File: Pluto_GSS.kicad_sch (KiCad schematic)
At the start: 7 parts

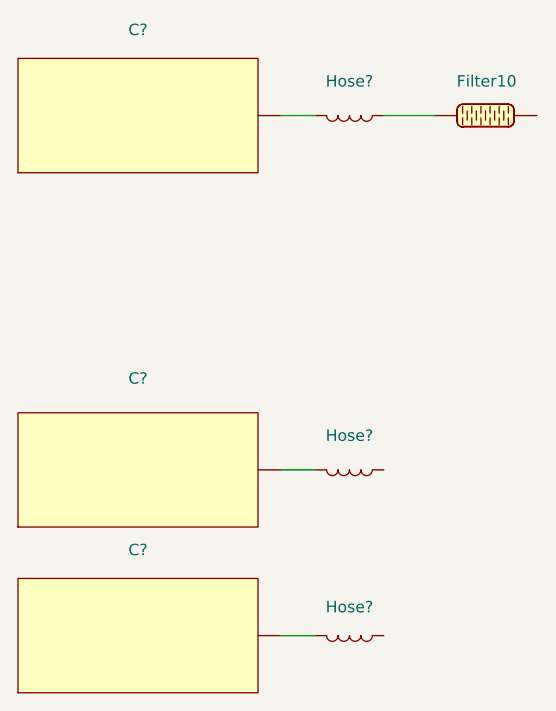
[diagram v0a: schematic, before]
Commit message: Formatiing
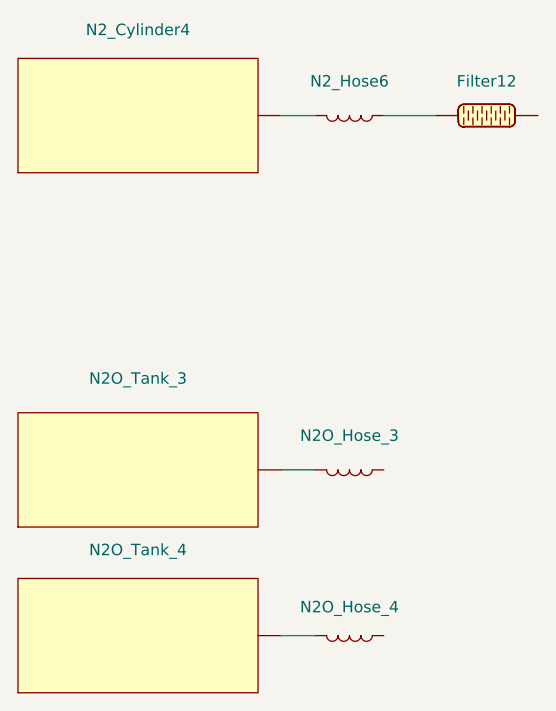
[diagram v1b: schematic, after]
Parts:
- gave numbers to parts that had none: 6
- renumbered Filter10 to Filter12
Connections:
- net at N2O_Hose_4.: now also N2O_Tank_4.
- net at Filter12.: now also N2_Hose6.
- net at N2_Hose6.: now also N2_Cylinder4.
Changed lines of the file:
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@@
 		(dnp no)
 		(fields_autoplaced yes)
-		(property "Reference" "C?"
+		(property "Reference" "N2O_Tank_3"
 			(at 77.47 93.98 90)
 			(effects
@@
 					(size 1.27 1.27)
 				)
-				(hide yes)
 			)
 		)
@@
 					(size 1.27 1.27)
 				)
-			)
-		)
-		(pin ""
-		)
-		(instances
-			(project "P_IDs"
-				(path "/045f1f05-3134-4b6d-91b6-463031104f1e/d4c68d07-3148-4b28-9ebc-772298248340/d1c23521-1854-4751-80d3-fa4616e29f0e"
-					(reference "C?")
-					(unit 1)
-				)
-			)
-		)
-	)
-	(symbol
+				(hide yes)
+			)
+		)
+		(pin ""
+		)
+		(instances
+			(project "P_IDs"
+				(path "/045f1f05-3134-4b6d-91b6-463031104f1e/d4c68d07-3148-4b28-9ebc-772298248340/d1c23521-1854-4751-80d3-fa4616e29f0e"
+					(reference "N2O_Tank_3")
+					(unit 1)
+				)
+			)
+		)
+	)
+	(symbol
+		(lib_name "Hose_1")
 		(lib_id "PID_symbols:Hose")
 		(at 97.155 122.555 270)
@@
 		(dnp no)
 		(fields_autoplaced yes)
-		(property "Reference" "Hose?"
+		(property "Reference" "N2O_Hose_4"
 			(at 100.965 119.38 90)
 			(effects
@@
 					(size 1.27 1.27)
 				)
-				(hide yes)
 			)
 		)
@@
 					(size 1.27 1.27)
 				)
-			)
-		)
-		(pin ""
-		)
-		(pin ""
-		)
-		(instances
-			(project "P_IDs"
-				(path "/045f1f05-3134-4b6d-91b6-463031104f1e/d4c68d07-3148-4b28-9ebc-772298248340/d1c23521-1854-4751-80d3-fa4616e29f0e"
-					(reference "Hose?")
+				(hide yes)
+			)
+		)
+		(pin ""
+		)
+		(pin ""
+		)
+		(instances
+			(project "P_IDs"
+				(path "/045f1f05-3134-4b6d-91b6-463031104f1e/d4c68d07-3148-4b28-9ebc-772298248340/d1c23521-1854-4751-80d3-fa4616e29f0e"
+					(reference "N2O_Hose_4")
 					(unit 1)
 				)
@@
 		(on_board yes)
 		(dnp no)
-		(property "Reference" "Filter10"
+		(property "Reference" "Filter12"
 			(at 116.205 60.96 0)
 			(effects
@@
 					(size 1.27 1.27)
 				)
-				(hide yes)
 			)
 		)
@@
 					(size 1.27 1.27)
 				)
-			)
-		)
-		(pin ""
-		)
-		(pin ""
-		)
-		(instances
-			(project "P_IDs"
-				(path "/045f1f05-3134-4b6d-91b6-463031104f1e/d4c68d07-3148-4b28-9ebc-772298248340/d1c23521-1854-4751-80d3-fa4616e29f0e"
-					(reference "Filter10")
+				(hide yes)
+			)
+		)
+		(pin ""
+		)
+		(pin ""
+		)
+		(instances
+			(project "P_IDs"
+				(path "/045f1f05-3134-4b6d-91b6-463031104f1e/d4c68d07-3148-4b28-9ebc-772298248340/d1c23521-1854-4751-80d3-fa4616e29f0e"
+					(reference "Filter12")
 					(unit 1)
 				)
@@
 		(dnp no)
 		(fields_autoplaced yes)
-		(property "Reference" "C?"
+		(property "Reference" "N2O_Tank_4"
 			(at 77.47 113.03 90)
 			(effects
@@
 					(size 1.27 1.27)
 				)
-				(hide yes)
 			)
 		)
@@
 					(size 1.27 1.27)
 				)
-			)
-		)
-		(pin ""
-		)
-		(instances
-			(project "P_IDs"
-				(path "/045f1f05-3134-4b6d-91b6-463031104f1e/d4c68d07-3148-4b28-9ebc-772298248340/d1c23521-1854-4751-80d3-fa4616e29f0e"
-					(reference "C?")
-					(unit 1)
-				)
-			)
-		)
-	)
-	(symbol
-		(lib_name "Hose_1")
+				(hide yes)
+			)
+		)
+		(pin ""
+		)
+		(instances
+			(project "P_IDs"
+				(path "/045f1f05-3134-4b6d-91b6-463031104f1e/d4c68d07-3148-4b28-9ebc-772298248340/d1c23521-1854-4751-80d3-fa4616e29f0e"
+					(reference "N2O_Tank_4")
+					(unit 1)
+				)
+			)
+		)
+	)
+	(symbol
 		(lib_id "PID_symbols:Hose")
 		(at 97.155 104.14 270)
@@
 		(dnp no)
 		(fields_autoplaced yes)
-		(property "Reference" "Hose?"
+		(property "Reference" "N2O_Hose_3"
 			(at 100.965 100.33 90)
 			(effects
@@
 					(size 1.27 1.27)
 				)
-				(hide yes)
 			)
 		)
@@
 					(size 1.27 1.27)
 				)
-			)
-		)
-		(pin ""
-		)
-		(pin ""
-		)
-		(instances
-			(project "P_IDs"
-				(path "/045f1f05-3134-4b6d-91b6-463031104f1e/d4c68d07-3148-4b28-9ebc-772298248340/d1c23521-1854-4751-80d3-fa4616e29f0e"
-					(reference "Hose?")
+				(hide yes)
+			)
+		)
+		(pin ""
+		)
+		(pin ""
+		)
+		(instances
+			(project "P_IDs"
+				(path "/045f1f05-3134-4b6d-91b6-463031104f1e/d4c68d07-3148-4b28-9ebc-772298248340/d1c23521-1854-4751-80d3-fa4616e29f0e"
+					(reference "N2O_Hose_3")
 					(unit 1)
 				)
@@
 		(dnp no)
 		(fields_autoplaced yes)
-		(property "Reference" "Hose?"
+		(property "Reference" "N2_Hose6"
 			(at 100.965 60.96 90)
 			(effects
@@
 					(size 1.27 1.27)
 				)
-				(hide yes)
 			)
 		)
@@
 					(size 1.27 1.27)
 				)
-			)
-		)
-		(pin ""
-		)
-		(pin ""
-		)
-		(instances
-			(project "P_IDs"
-				(path "/045f1f05-3134-4b6d-91b6-463031104f1e/d4c68d07-3148-4b28-9ebc-772298248340/d1c23521-1854-4751-80d3-fa4616e29f0e"
-					(reference "Hose?")
+				(hide yes)
+			)
+		)
+		(pin ""
+		)
+		(pin ""
+		)
+		(instances
+			(project "P_IDs"
+				(path "/045f1f05-3134-4b6d-91b6-463031104f1e/d4c68d07-3148-4b28-9ebc-772298248340/d1c23521-1854-4751-80d3-fa4616e29f0e"
+					(reference "N2_Hose6")
 					(unit 1)
 				)
@@
 		(dnp no)
 		(fields_autoplaced yes)
-		(property "Reference" "C?"
+		(property "Reference" "N2_Cylinder4"
 			(at 77.47 55.245 90)
 			(effects
@@
 					(size 1.27 1.27)
 				)
-				(hide yes)
 			)
 		)
@@
 					(size 1.27 1.27)
 				)
-			)
-		)
-		(pin ""
-		)
-		(instances
-			(project "P_IDs"
-				(path "/045f1f05-3134-4b6d-91b6-463031104f1e/d4c68d07-3148-4b28-9ebc-772298248340/d1c23521-1854-4751-80d3-fa4616e29f0e"
-					(reference "C?")
-					(unit 1)
-				)
+				(hide yes)
+			)
+		)
+		(pin ""
+		)
+		(instances
+			(project "P_IDs"
+				(path "/045f1f05-3134-4b6d-91b6-463031104f1e/d4c68d07-3148-4b28-9ebc-772298248340/d1c23521-1854-4751-80d3-fa4616e29f0e"
+					(reference "N2_Cylinder4")
+					(unit 1)
+				)
